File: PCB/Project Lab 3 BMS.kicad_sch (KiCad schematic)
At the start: 46 parts, among them J1 Conn_01x02, J3 Conn_01x06, Q1 IRLR7843, Q2 IRLR7843, Q3 PMOS, SW1 Start Swtich, U1 BQ76920PW, U2 ESP32-WROOM-32

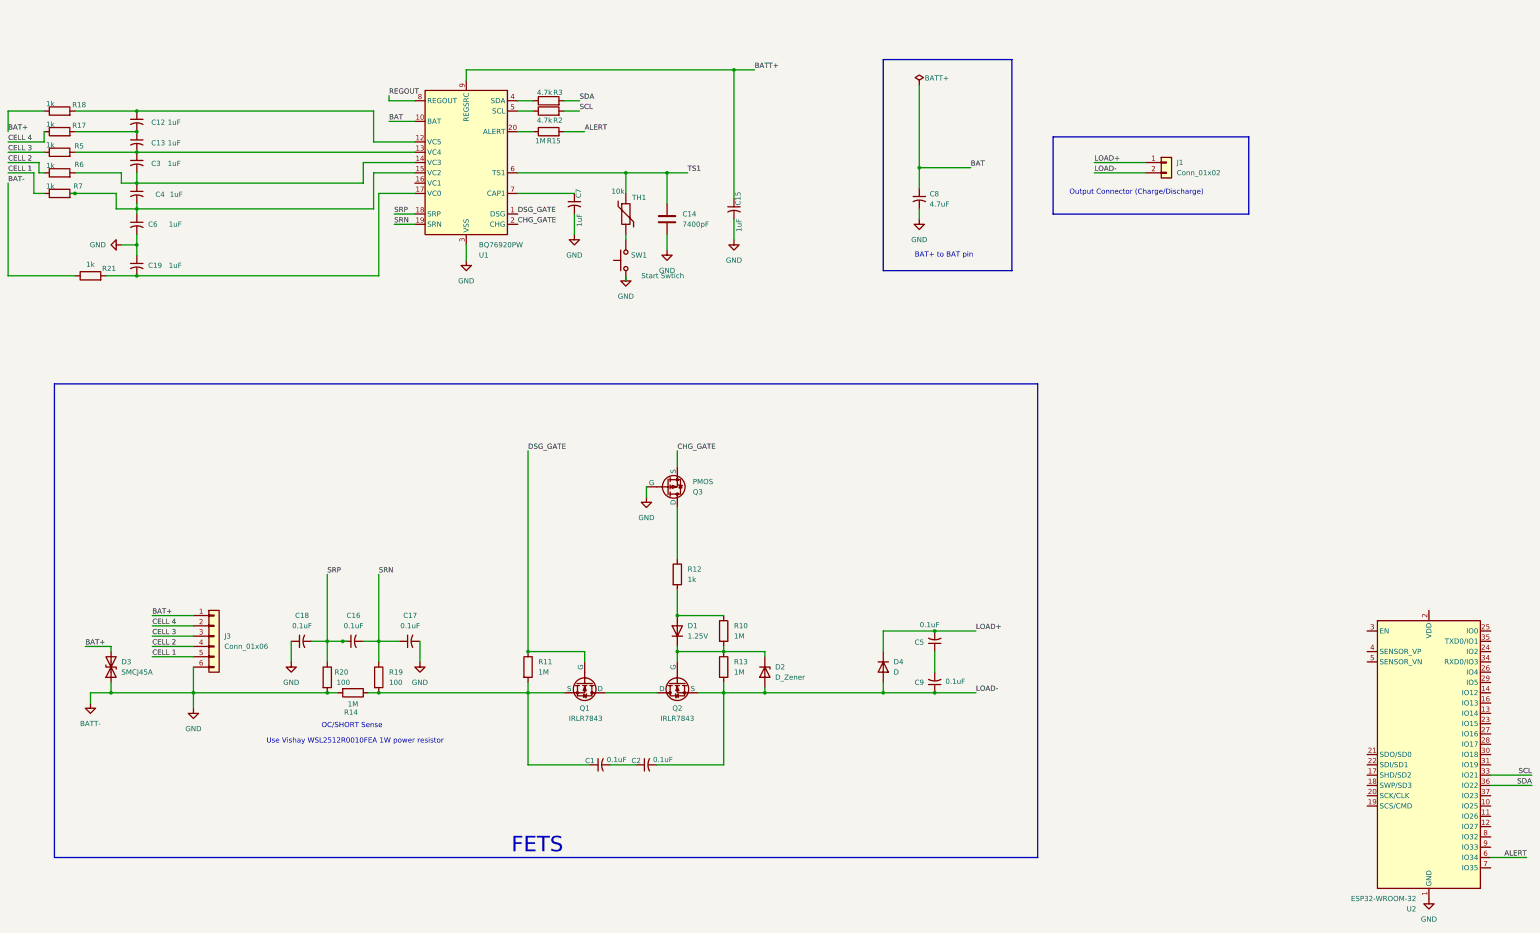
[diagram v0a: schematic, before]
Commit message: Footprints Assigned
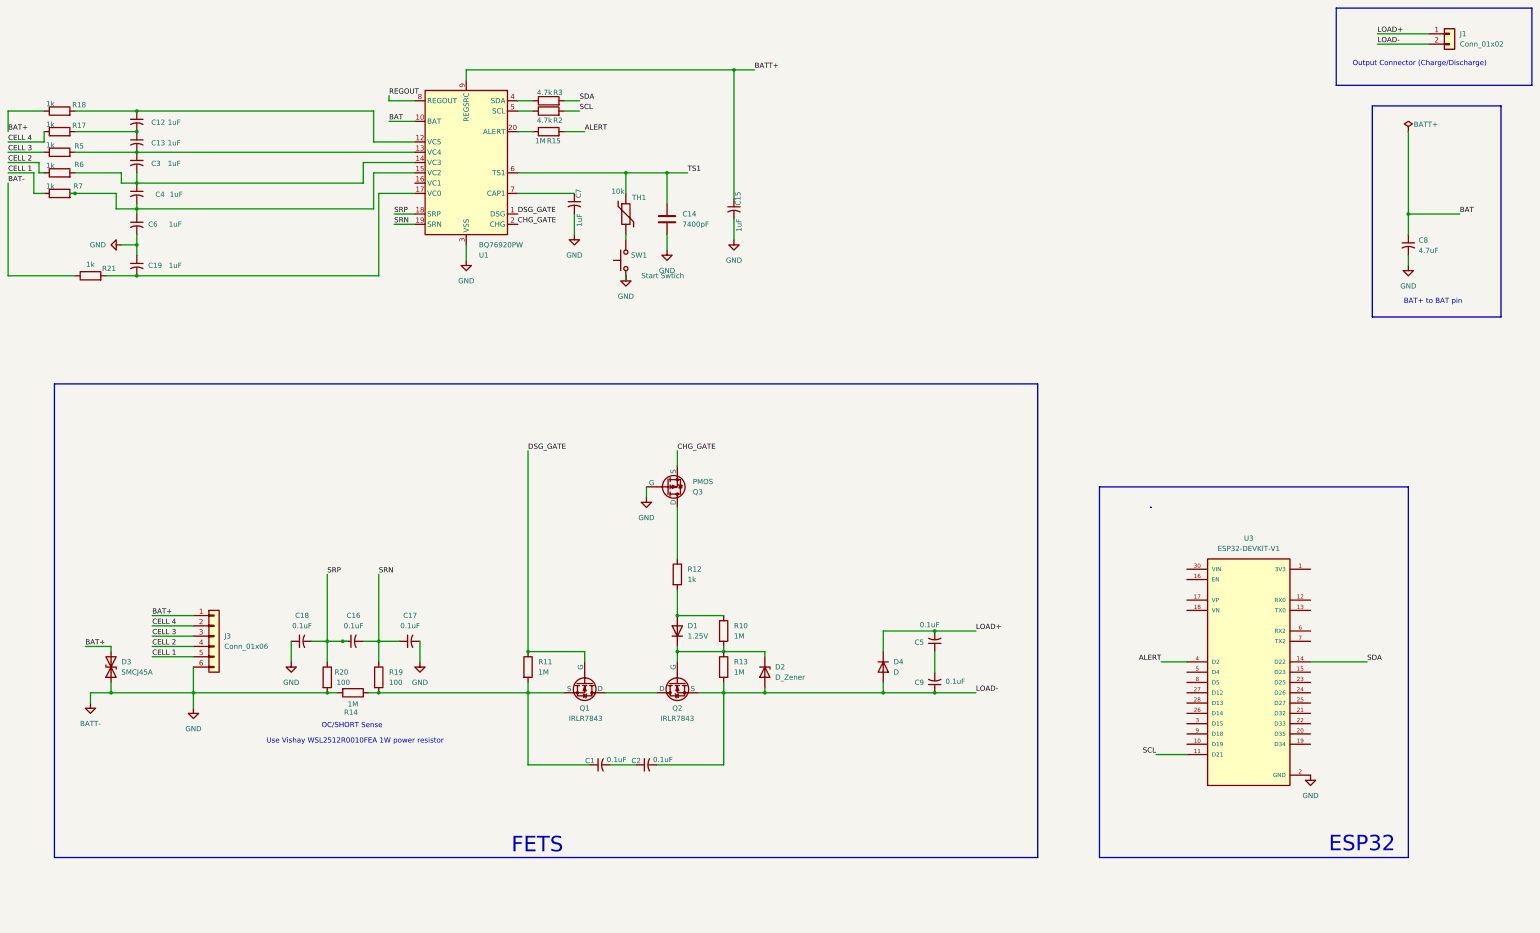
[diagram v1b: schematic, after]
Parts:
- removed U2: ESP32-WROOM-32, RF_Module:ESP32-WROOM-32, symbol RF_Module:ESP32-WROOM-32
- added U3: ESP32-DEVKIT-V1, Snapeda:MODULE_ESP32_DEVKIT_V1, symbol Snapeda:ESP32-DEVKIT-V1
- C1, C12, C13, C14, C15, C16, C17, C18, C19, C2, C3, C4, C5, C6, C7, C9, R2, R3, R5, R6, R7: footprint (none) -> Capacitor_SMD:C_0805_2012Metric
- C8: footprint (none) -> Capacitor_SMD:C_1206_3216Metric
- D1, D4: footprint (none) -> Diode_SMD:D_SOD-123
- D2: footprint (none) -> Diode_SMD:D_0201_0603Metric
- D3: footprint (none) -> Diode_SMD:D_SMC
- J1: footprint (none) -> TerminalBlock_Phoenix:TerminalBlock_Phoenix_MKDS-1,5-2_1x02_P5.00mm_Horizontal
- J3: footprint (none) -> Connector_JST:JST_XH_B6B-XH-A_1x06_P2.50mm_Vertical
- Q1, Q2, Q3: footprint (none) -> Package_TO_SOT_SMD:TO-252-2
- R10, R11, R12, R13, R14, R15: footprint (none) -> Resistor_SMD:R_2512_6332Metric
- R17, R18, R19, R20, R21, TH1: footprint (none) -> Resistor_SMD:R_0805_2012Metric
- SW1: footprint (none) -> Button_Switch_SMD:SW_SPST_PTS645Sx43SMTR92
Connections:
- net ALERT: now also U3.4 (D2)
- net BATT-: now also U3.2 (GND), U3.29 (GND)
- net SCL: now also U3.11 (D21)
- net SDA: now also U3.14 (D22)
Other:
- note added: "ESP32"
- moved on the sheet: C8, J1
